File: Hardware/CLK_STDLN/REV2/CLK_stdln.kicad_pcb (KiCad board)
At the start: 2 copper layers, 63.9 x 67 mm, 43 parts, among them J1 Conn_01x04_Male, J2 Conn_Coaxial, J3 Conn_01x02, J4 Conn_02x20_Counter_Clockwise, Q1 BC547, Q2 BC547, Q3 BC547, SW1 SW_Push, SW2 SW_SPDT, SW3 SW_SPDT, U1 74LS08, U2 74LS04, U3 NE555, U4 NE555, U5 NE555

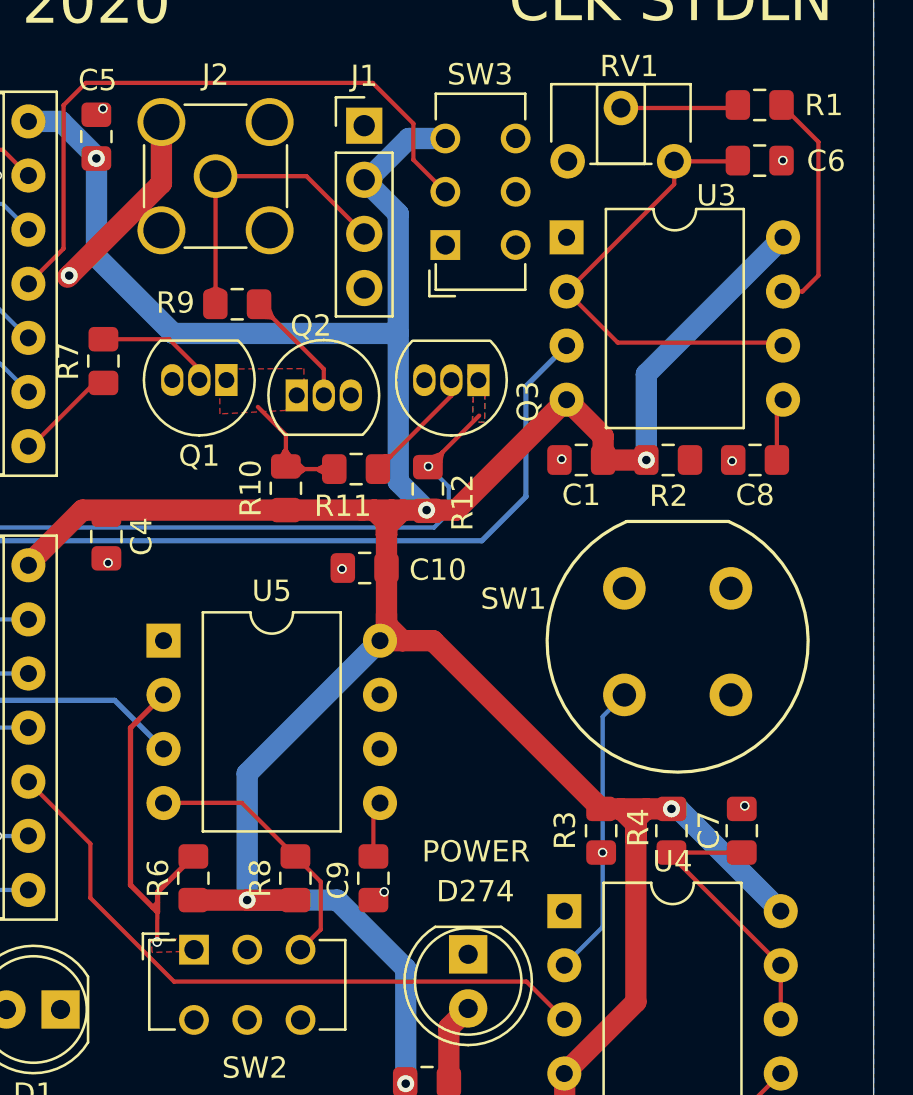
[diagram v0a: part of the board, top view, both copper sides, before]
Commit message: 0041 | 0,1h | review STDLN CLK REV 2
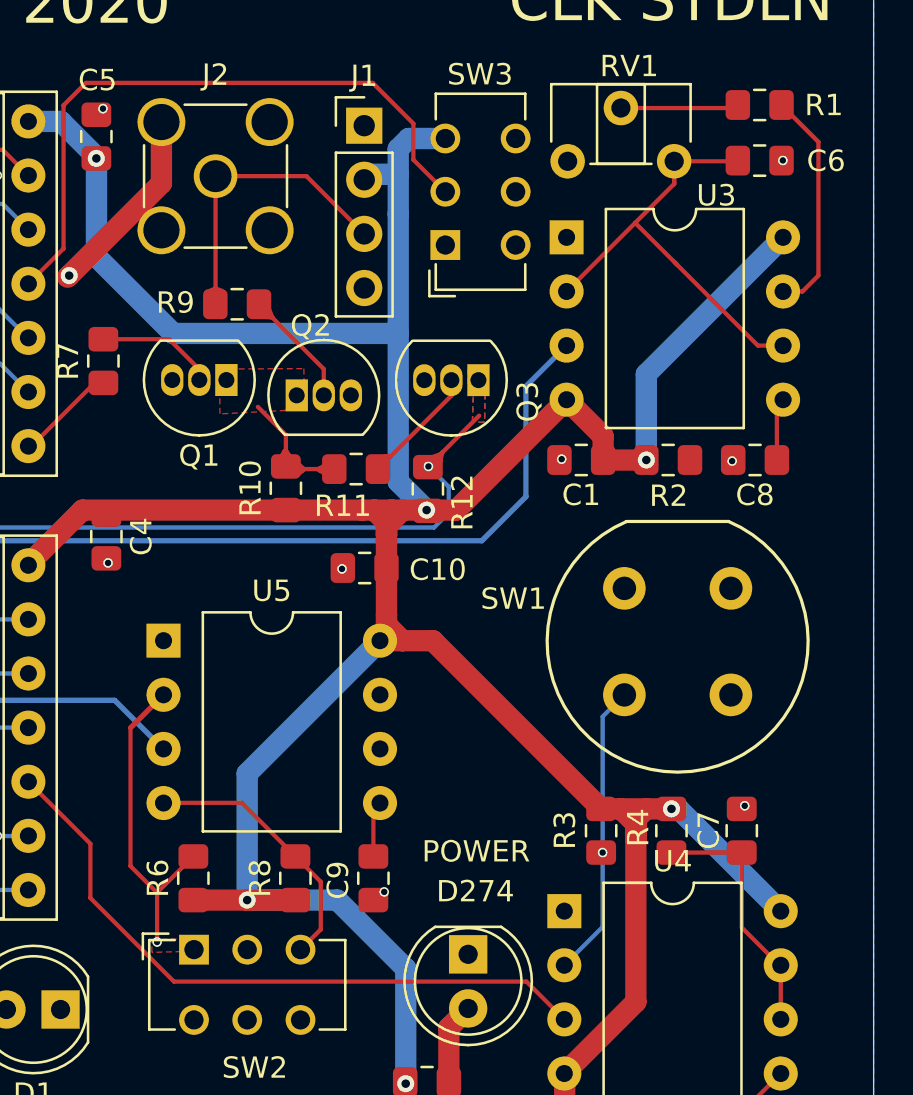
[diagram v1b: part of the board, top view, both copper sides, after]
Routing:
- net Net-(R6-Pad2): track 16.5 -> 15.3 mm
- net Net-(C7-Pad1): track 14.3 -> 13.2 mm
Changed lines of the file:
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@@
     (thickness 1.6)
     (drawings 5)
-    (tracks 318)
+    (tracks 321)
     (modules 43)
     (nets 69)
@@
   )
   (gr_rect (start 209.31 153.54) (end 145.36 86.52) (layer "Edge.Cuts") (width 0.05))
+  (segment (start 204.952 134.864) (end 204.894 134.864) (width 0.2) (layer "F.Cu") (net 5))
+  (segment (start 204.894 134.864) (end 203.122 133.092) (width 0.2) (layer "F.Cu") (net 5))
+  (segment (start 203.122 133.092) (end 203.122 129.574) (width 0.2) (layer "F.Cu") (net 5))
+  (segment (start 174.4325 123.72) (end 174.4325 130.20776) (width 0.2) (layer "F.Cu") (net 52))
+  (segment (start 174.4325 130.20776) (end 175.68112 131.45638) (width 0.2) (layer "F.Cu") (net 52))
+  (segment (start 175.68112 133.77112) (end 175.68112 131.45638) (width 0.2) (layer "F.Cu") (net 52))
+  (segment (start 175.68112 131.45638) (end 177.3825 129.755) (width 0.2) (layer "F.Cu") (net 52))
+  (segment (start 203.88 105.78) (end 200.075 101.975) (width 0.2) (layer "F.Cu") (net 4))
+  (segment (start 200.075 101.975) (end 199.95 101.85) (width 0.2) (layer "F.Cu") (net 4))
+  (segment (start 194.9 103.24) (end 198.12 100.02) (width 0.2) (layer "F.Cu") (net 4))
+  (segment (start 200.075 101.975) (end 198.12 100.02) (width 0.2) (layer "F.Cu") (net 4))
+  (segment (start 198.12 100.02) (end 199.95 98.19) (width 0.2) (layer "F.Cu") (net 4))
+  (segment (start 199.95 98.19) (end 199.95 97.13) (width 0.2) (layer "F.Cu") (net 4))
+  (segment (start 205.06 105.78) (end 203.88 105.78) (width 0.2) (layer "F.Cu") (net 4))
+  (segment (start 186.99699 99.59299) (end 186.99699 97.74301) (width 1) (layer "B.Cu") (net 2))
+  (segment (start 185.65699 97.74301) (end 185.402 97.998) (width 1) (layer "B.Cu") (net 2))
+  (segment (start 186.99699 97.74301) (end 186.99699 96.55301) (width 1) (layer "B.Cu") (net 2))
+  (segment (start 186.99699 97.74301) (end 185.65699 97.74301) (width 1) (layer "B.Cu") (net 2))
+  (segment (start 186.99699 96.55301) (end 187.49 96.06) (width 1) (layer "B.Cu") (net 2))
   (segment (start 168.432 96.59) (end 157.55 96.59) (width 0.2) (layer "F.Cu") (net 41))
   (segment (start 169.64 97.798) (end 168.432 96.59) (width 0.2) (layer "F.Cu") (net 41))
@@
   (segment (start 179.9075 131.805) (end 184.135 131.805) (width 1) (layer "B.Cu") (net 2))
   (segment (start 187.35 135.02) (end 187.35 140.42) (width 1) (layer "B.Cu") (net 2))
-  (segment (start 175.6925 132.36) (end 175.68112 133.77112) (width 0.2) (layer "F.Cu") (net 52))
   (segment (start 172.34 93.45) (end 171.29 94.5) (width 0.2) (layer "F.Cu") (net 56))
   (segment (start 185.8 93.45) (end 172.34 93.45) (width 0.2) (layer "F.Cu") (net 56))
@@
   (segment (start 189.719 113.501) (end 194.9 108.32) (width 1) (layer "F.Cu") (net 2))
   (segment (start 188.33 113.501) (end 189.719 113.501) (width 1) (layer "F.Cu") (net 2))
-  (segment (start 175.7025 132.36) (end 175.7025 131.9075) (width 0.25) (layer "F.Cu") (net 52))
-  (segment (start 175.47625 132.14375) (end 174.4325 131.1) (width 0.25) (layer "F.Cu") (net 52))
-  (segment (start 175.7025 131.9075) (end 175.7025 131.435) (width 0.25) (layer "F.Cu") (net 52))
-  (segment (start 175.47625 132.13375) (end 175.7025 131.9075) (width 0.2) (layer "F.Cu") (net 52))
-  (segment (start 175.6925 132.36) (end 175.47625 132.14375) (width 0.25) (layer "F.Cu") (net 52))
-  (segment (start 175.47625 132.14375) (end 175.47625 132.13375) (width 0.2) (layer "F.Cu") (net 52))
   (segment (start 174.4325 123.72) (end 175.9825 122.17) (width 0.25) (layer "F.Cu") (net 52))
-  (segment (start 175.7025 131.435) (end 177.3825 129.755) (width 0.25) (layer "F.Cu") (net 52))
-  (segment (start 175.7025 132.36) (end 175.6925 132.36) (width 0.25) (layer "F.Cu") (net 52))
-  (segment (start 174.4325 131.1) (end 174.4325 123.72) (width 0.25) (layer "F.Cu") (net 52))
   (segment (start 194.9 105.78) (end 194.9 105.85) (width 0.2) (layer "B.Cu") (net 66))
   (segment (start 169.64 116.04) (end 172.179 113.501) (width 1) (layer "F.Cu") (net 2))
@@
   (segment (start 172.55 131.704502) (end 172.55 129.16) (width 0.2) (layer "F.Cu") (net 61))
   (segment (start 172.55 129.16) (end 169.64 126.25) (width 0.2) (layer "F.Cu") (net 61))
-  (segment (start 185.552 97.998) (end 187.49 96.06) (width 1) (layer "B.Cu") (net 2))
   (segment (start 185.402 97.998) (end 185.552 97.998) (width 1) (layer "B.Cu") (net 2))
   (segment (start 187.49 96.06) (end 189.21 96.06) (width 1) (layer "B.Cu") (net 2))
@@
   (segment (start 186.99699 112.16799) (end 186.99699 105.20901) (width 1) (layer "B.Cu") (net 2))
   (segment (start 188.33 113.501) (end 186.99699 112.16799) (width 1) (layer "B.Cu") (net 2))
-  (segment (start 186.99699 99.59299) (end 185.402 97.998) (width 1) (layer "B.Cu") (net 2))
   (via (at 188.33 113.501) (size 0.8) (drill 0.4) (layers "F.Cu" "B.Cu") (net 2))
   (segment (start 173.16 107.531) (end 172.755 107.531) (width 0.2) (layer "F.Cu") (net 53))
@@
   (segment (start 204.952 134.864) (end 204.952 137.404) (width 0.2) (layer "F.Cu") (net 5))
   (segment (start 199.822 129.574) (end 199.822 129.734) (width 0.2) (layer "F.Cu") (net 5))
-  (segment (start 199.822 129.734) (end 204.952 134.864) (width 0.2) (layer "F.Cu") (net 5))
   (segment (start 204.932 134.864) (end 204.952 134.864) (width 0.2) (layer "B.Cu") (net 5))
   (segment (start 199.822 129.574) (end 203.122 129.574) (width 0.2) (layer "F.Cu") (net 5))
@@
   (segment (start 182.1725 129.755) (end 179.6575 127.24) (width 0.2) (layer "F.Cu") (net 54))
   (segment (start 175.9925 127.24) (end 175.9825 127.25) (width 0.2) (layer "F.Cu") (net 54))
-  (segment (start 194.92 103.24) (end 199.95 98.21) (width 0.2) (layer "F.Cu") (net 4))
   (segment (start 194.9 103.24) (end 194.92 103.24) (width 0.2) (layer "F.Cu") (net 4))
   (segment (start 199.95 98.21) (end 199.95 97.13) (width 0.2) (layer "F.Cu") (net 4))
-  (segment (start 204.92 105.64) (end 197.3 105.64) (width 0.2) (layer "F.Cu") (net 4))
   (segment (start 205.06 105.78) (end 204.92 105.64) (width 0.2) (layer "F.Cu") (net 4))
-  (segment (start 197.3 105.64) (end 194.9 103.24) (width 0.2) (layer "F.Cu") (net 4))
   (segment (start 183.3625 133.18) (end 183.3625 130.945) (width 0.2) (layer "F.Cu") (net 54))
   (segment (start 182.4125 134.13) (end 183.3625 133.18) (width 0.2) (layer "F.Cu") (net 54))
